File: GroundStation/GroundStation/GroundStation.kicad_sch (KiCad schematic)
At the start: 72 parts, among them J1 SD_Card_Receptacle, J4 Conn_Coaxial, J5 Conn_01x02, P1 USB_C_Plug_USB2.0, Q1 TSM3481CX6 RFG, U1 STM32F103C8Tx, U10 E22-400T30S, U101 LD1117S33TR_SOT223, U11 E80-900M23313S, U4 TPS54538RQFR, U9 NEO-M9N-00B

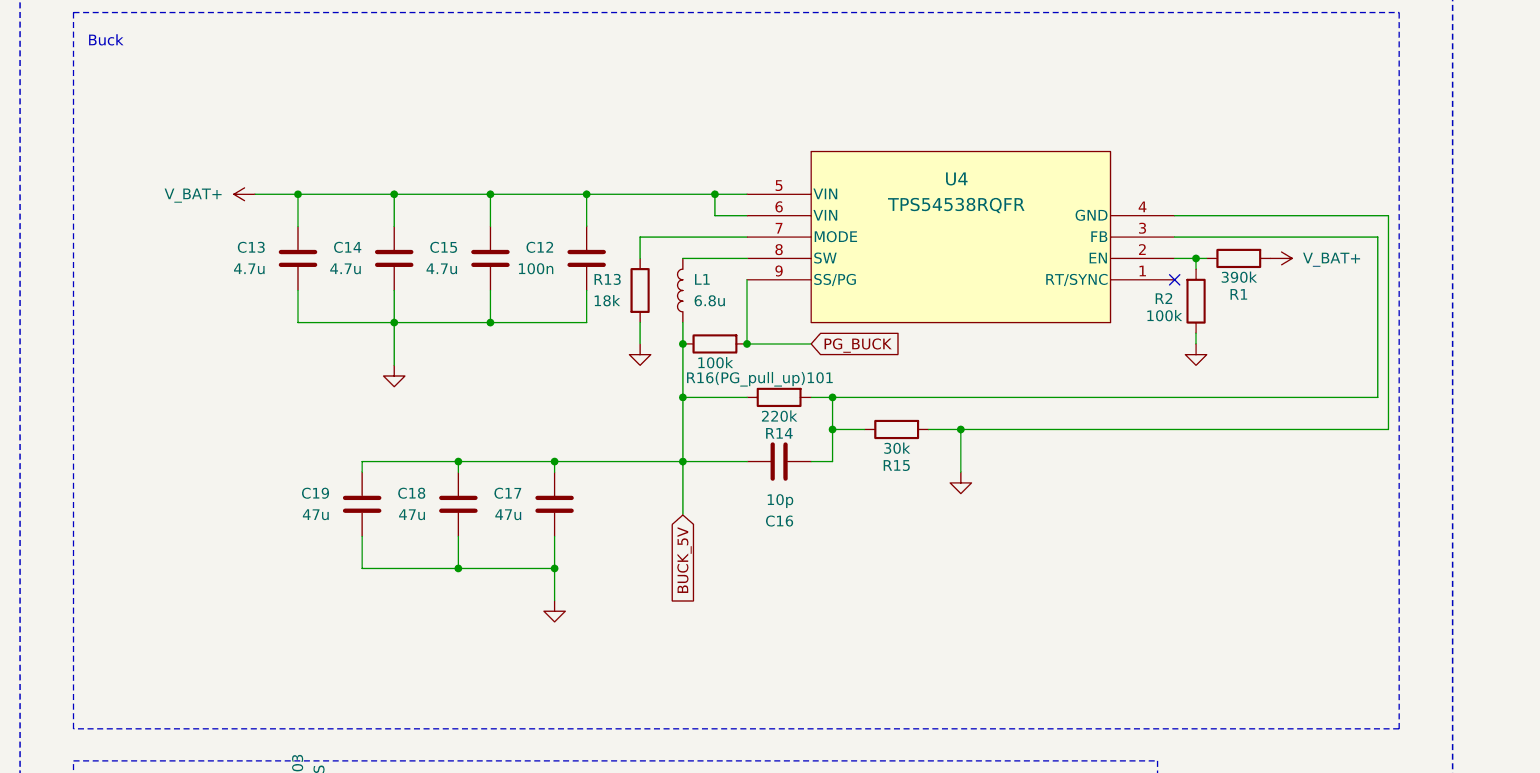
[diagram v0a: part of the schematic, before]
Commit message: second need freerouting
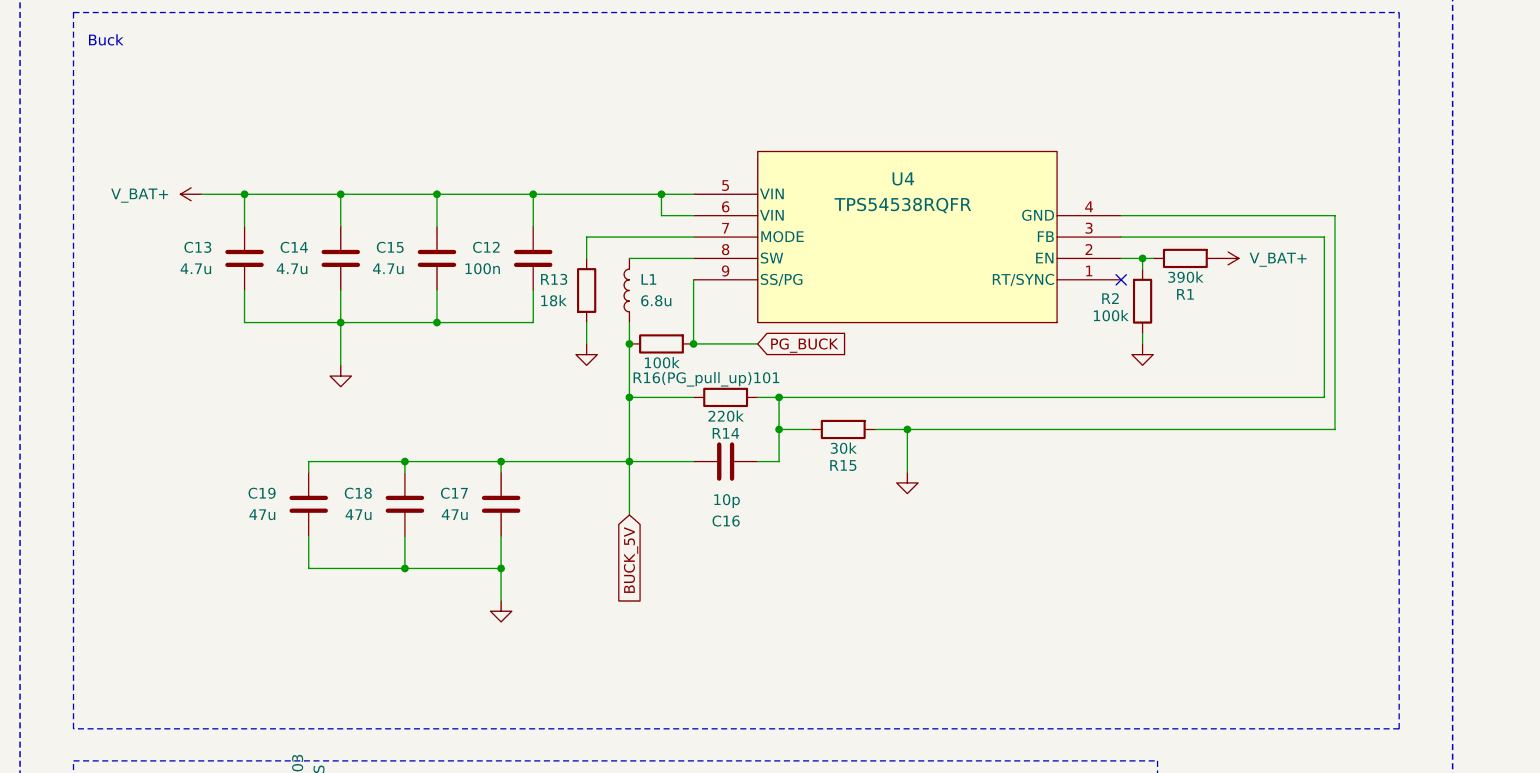
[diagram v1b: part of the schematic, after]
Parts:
- P1: footprint Connector_USB:USB3_A_Molex_48393-001 -> Connector_USB:USB_C_Receptacle_JAE_DX07S016JA1R1500
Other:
- moved on the sheet: C12, C13, C14, C15, C16, C17, C18, C19, L1, R1, R13, R14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
